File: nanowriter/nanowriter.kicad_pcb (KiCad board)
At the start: 2 copper layers, 19 parts, among them IC1 ATMEGA32U2, J1 USB_mini_micro_B, K1 KEYSW, K2 KEYSW, K3 KEYSW, K4 KEYSW, K5 KEYSW, K6 KEYSW, SW1 SW_PUSH, X1 XTAL_GND

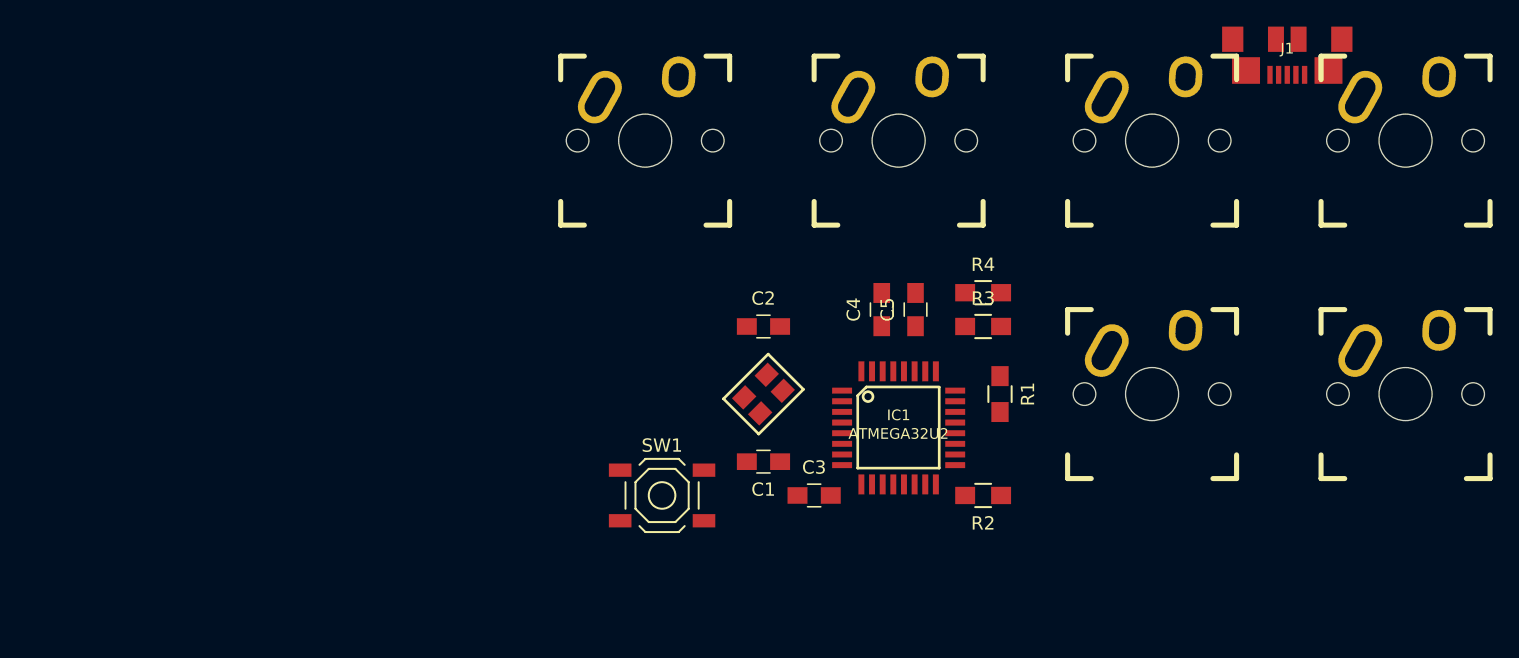
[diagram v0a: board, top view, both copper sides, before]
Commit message: Rev 1 pcb
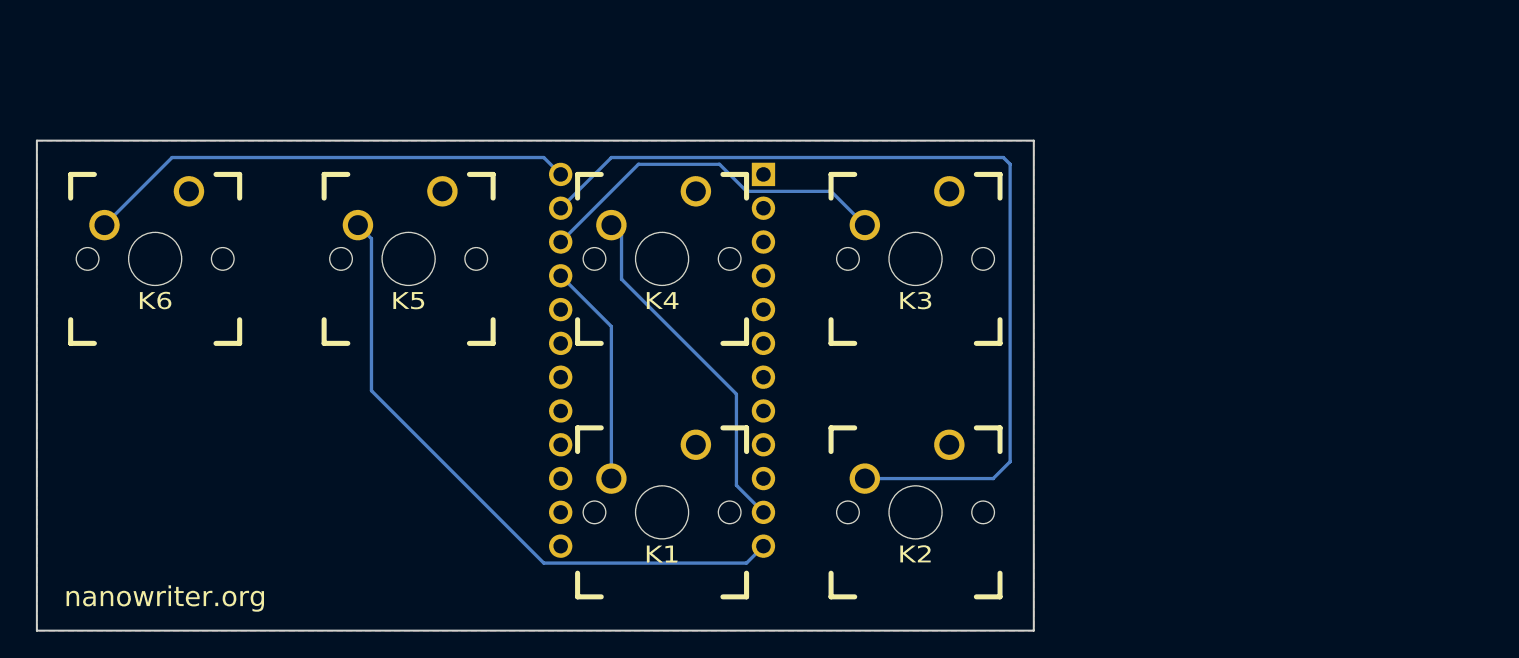
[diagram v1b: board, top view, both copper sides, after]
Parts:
- removed C1, C2: 22p, Capacitors_SMD:C_0805_HandSoldering
- removed C3: 0.1u, Capacitors_SMD:C_0805_HandSoldering
- removed C4: 4.7u, Capacitors_SMD:C_0805_HandSoldering
- removed C5: 1u, Capacitors_SMD:C_0805_HandSoldering
- removed IC1: ATMEGA32U2, keyboard_parts:QFP32
- removed J1: USB_mini_micro_B, keyboard_parts:USB_microB
- removed R1, R2: 10k, Resistors_SMD:R_0805_HandSoldering
- removed R3, R4: 22, Resistors_SMD:R_0805_HandSoldering
- removed SW1: SW_PUSH, Buttons_Switches_SMD:SW_SPST_TL3342
- removed X1: XTAL_GND, keyboard_parts:FA-238
- added U1: ProMicro, keebs:Pro_Micro, B.Cu at (134.6, 96.5)
- K1, K2, K3, K4, K5, K6: footprint keebs:Mx_Alps_100 -> Keyboard:CHERRY_PCB_100H
- moved K2 37.9 mm to (153.7, 108.0)
- moved K3 37.9 mm to (153.7, 88.9)
- moved K5 37.9 mm to (115.6, 88.9)
- moved K6 37.9 mm to (96.5, 88.9)
- moved K1 37.9 mm to (134.6, 108.0)
- moved K4 37.9 mm to (134.6, 88.9)
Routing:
- net Net-(K2-Pad2): track 0.00 -> 69.4 mm
- net Net-(K5-Pad2): track 0.00 -> 48.2 mm
- net Net-(K6-Pad2): track 0.00 -> 36.9 mm
- net Net-(K3-Pad2): track 0.00 -> 27.2 mm
- net Net-(K4-Pad2): track 0.00 -> 26.3 mm
- net Net-(K1-Pad2): track 0.00 -> 16.8 mm
- added copper zone on B.Cu, net GND
- added copper zone on F.Cu, net GND
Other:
- board outline added: 74.9 x 36.8 mm
- board text added: "nanowriter.org"
